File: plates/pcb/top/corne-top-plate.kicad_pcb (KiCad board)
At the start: 2 copper layers, 132.9 x 91.4 mm, 28 parts, among them SW2 KEY_SWITCH

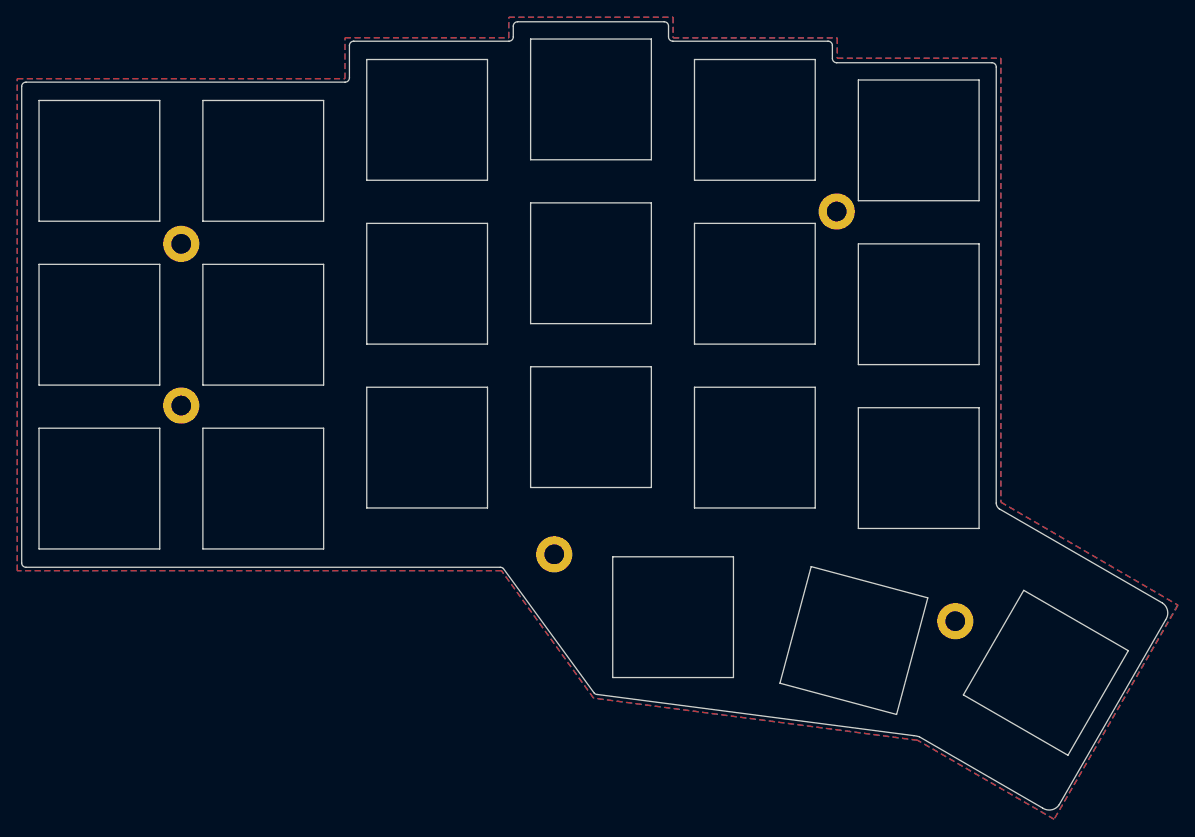
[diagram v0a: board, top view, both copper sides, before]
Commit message: plates
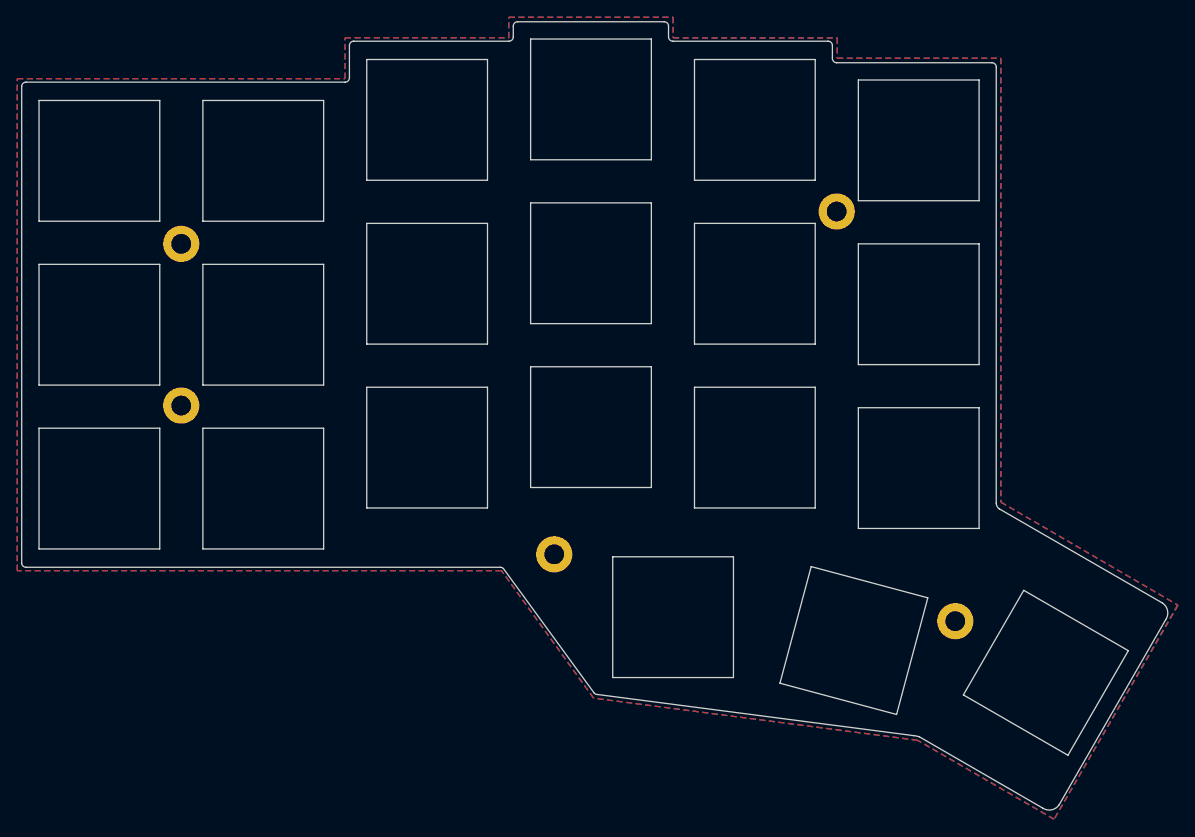
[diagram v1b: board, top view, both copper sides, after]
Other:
- net class Default removed
